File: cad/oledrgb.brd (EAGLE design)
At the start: 27.5 x 29.5 mm, 17 parts, among them U1 FAN5331SX

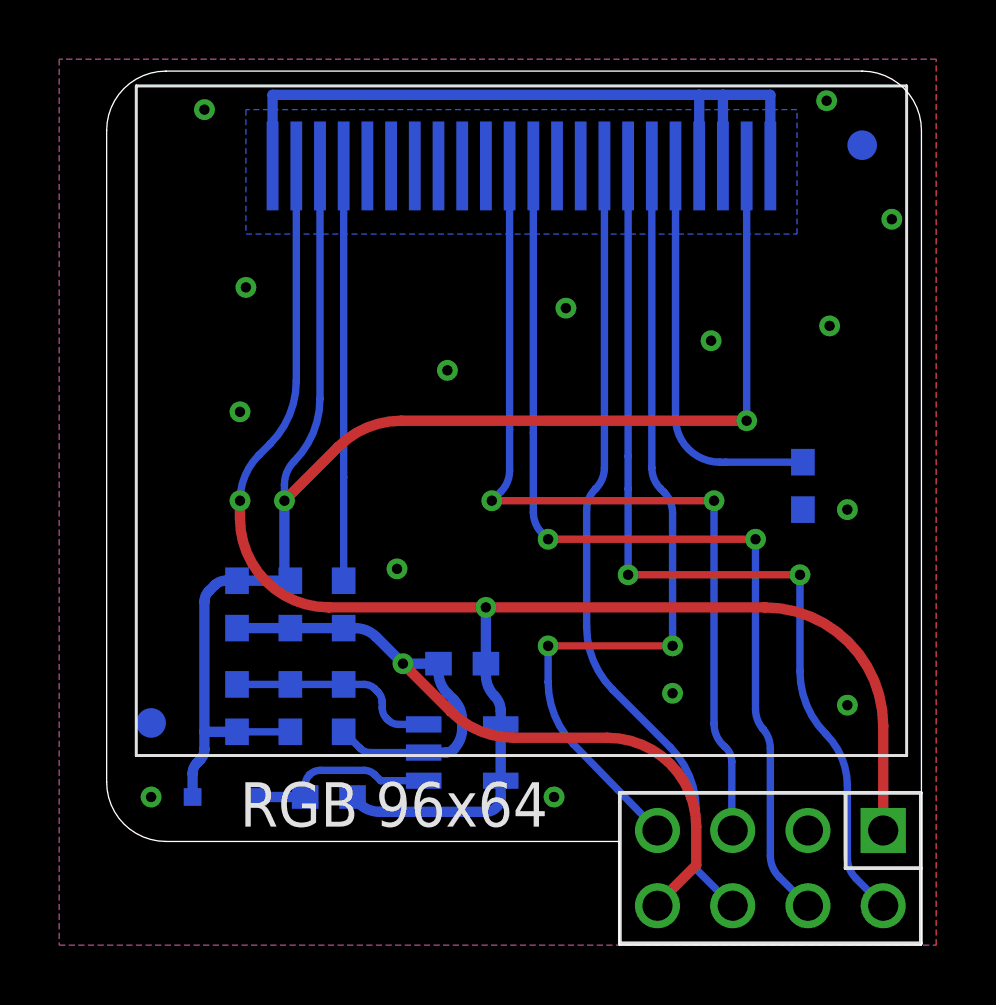
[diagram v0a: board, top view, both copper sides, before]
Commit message: embiggen connector
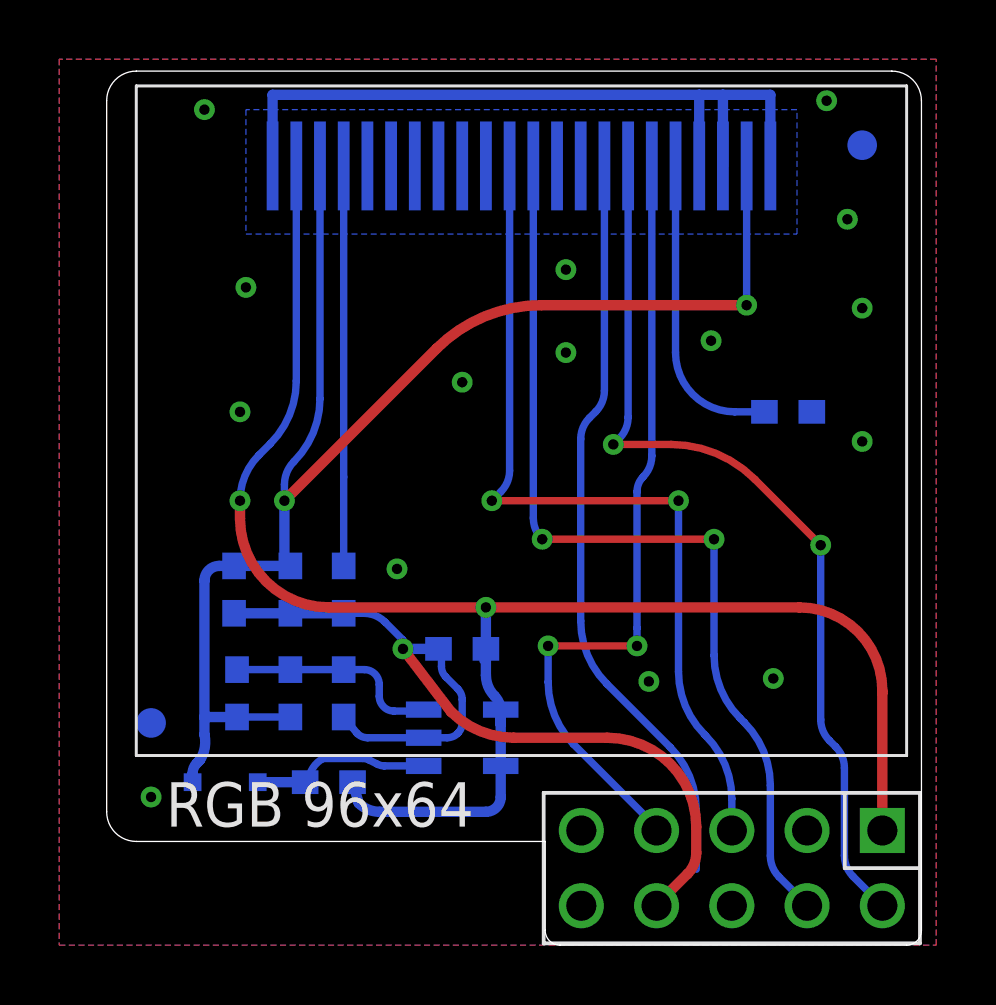
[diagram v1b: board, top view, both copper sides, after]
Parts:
- removed CN1: (no value), jaw:HEADER-2X04
- added CONN2: HEADER-5X2-PTH, jaw:HEADER-5X2-PTH
- moved R3 2.55 mm to (59.0, 18.5), turned to 180 degrees
- moved C5 0.51 mm to (40.3, 12.5)
- moved C1 0.50 mm to (48.0, 10.5)
- moved C2 0.50 mm to (40.4, 9.00)
- moved C3 0.50 mm to (42.2, 12.5)
- moved C4 0.50 mm to (44.0, 12.5)
- moved D1 0.50 mm to (40.0, 6.00)
- moved L1 0.50 mm to (43.5, 6.00)
- moved R1 0.50 mm to (42.2, 9.00)
- moved R2 0.50 mm to (44.0, 9.00)
- moved U1 0.50 mm to (48.0, 7.50)
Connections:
- new net N$19: CONN2.10
- new net N$4: CONN2.9
- net DPYCS: now also CONN2.7; no longer CN1.7
- net DPYDC: now also CONN2.6; no longer CN1.6
- net GND: now also CONN2.8; no longer CN1.8
- net NRST: now also CONN2.2; no longer CN1.2
- net SPIMISO: now also CONN2.3; no longer CN1.3
- net SPIMOSI: now also CONN2.5; no longer CN1.5
- net SPISCK: now also CONN2.4; no longer CN1.4
- net VCC: now also CONN2.1; no longer CN1.1
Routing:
- net N$20: track 13.4 -> 10.1 mm
- net V12: track 52.2 -> 49.4 mm
- net VCC: track 52.5 -> 54.9 mm
- net DPYDC: track 26.8 -> 25.2 mm
- net DPYCS: track 28.1 -> 26.9 mm
- net SPIMOSI: track 30.3 -> 29.3 mm
- net NRST: track 31.5 -> 30.5 mm
- net SPISCK: track 32.7 -> 31.7 mm
- net GND: track 55.9 -> 56.7 mm
- net N$6: track 14.0 -> 13.5 mm
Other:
- outline, holes or cut-outs redrawn
